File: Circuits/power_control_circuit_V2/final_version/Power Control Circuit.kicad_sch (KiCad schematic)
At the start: 41 parts, among them Q10 IRF1405, Q12 IRF1405, Q23 S8050, Q24 S8550, Q3 S8050, Q4 IRF1405, Q4 S8550, Q8 IRF1405, Q9 IRF1405, U1 PC817, U2 PC817

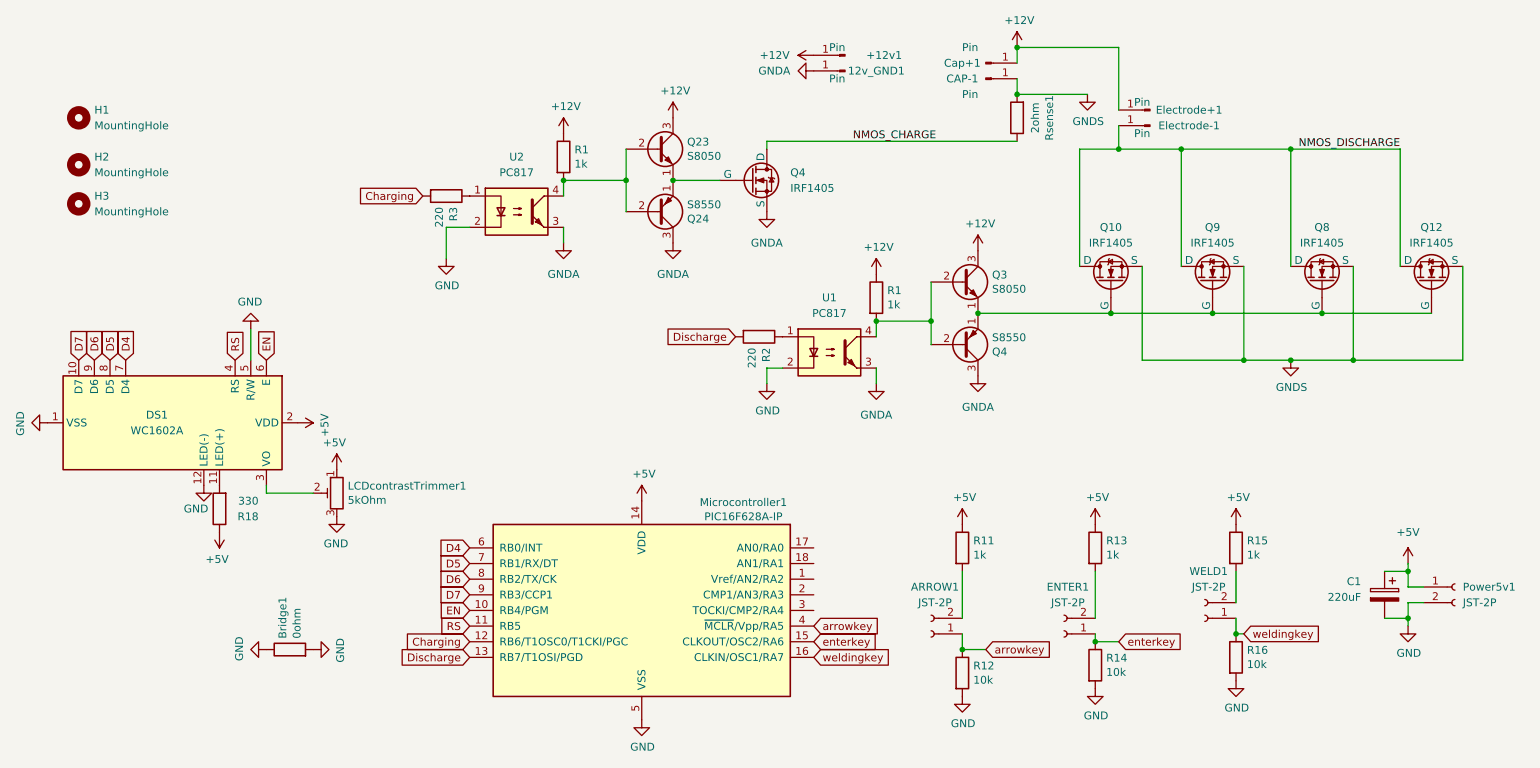
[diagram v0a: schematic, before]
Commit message: minor changes
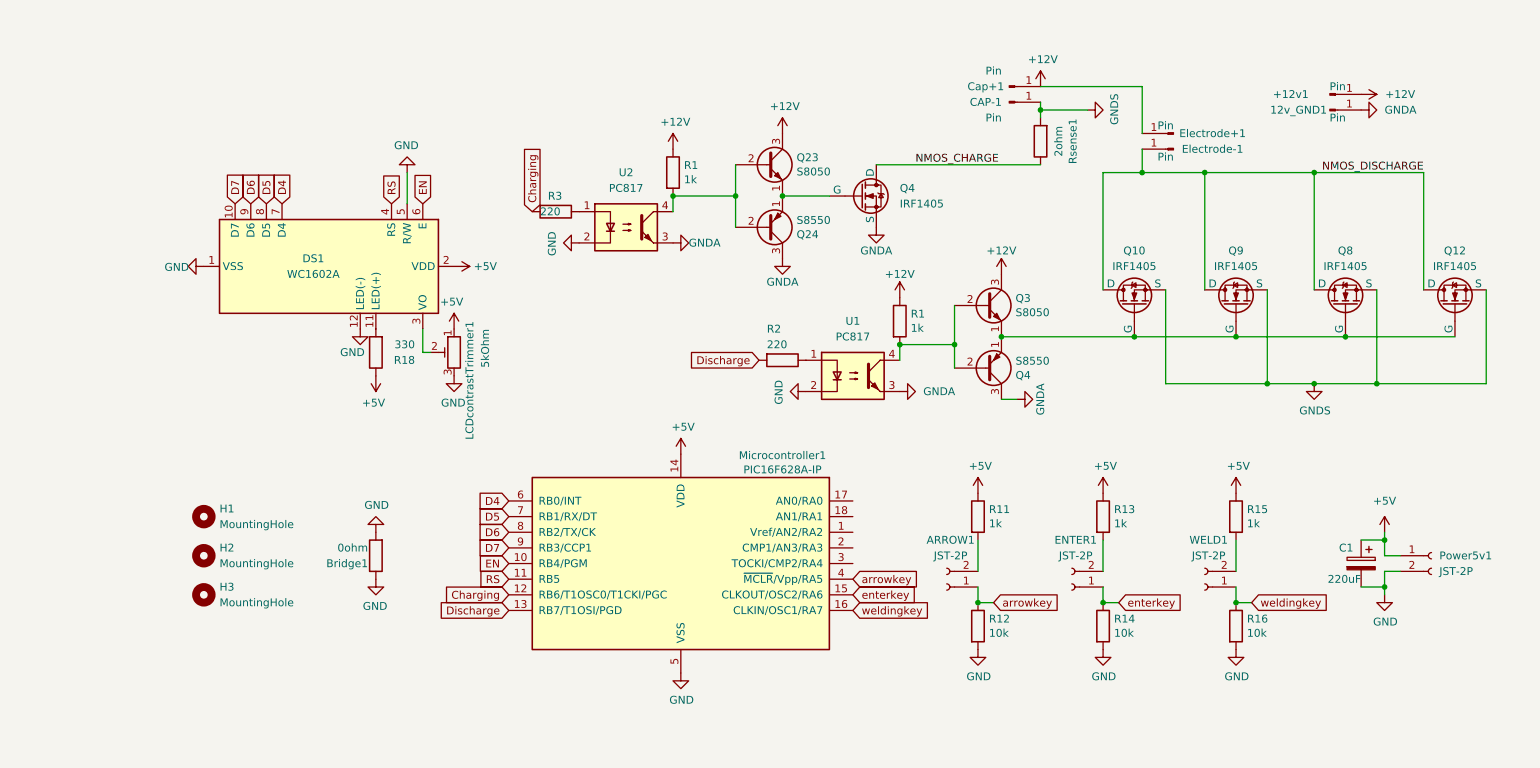
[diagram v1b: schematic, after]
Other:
- moved on the sheet: +12v1, 12v_GND1, ARROW1, Bridge1, C1, CAP-1, Cap+1, DS1, ENTER1, Electrode+1, Electrode-1, H1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
